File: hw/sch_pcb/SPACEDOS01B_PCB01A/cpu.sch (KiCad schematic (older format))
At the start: 27 parts, among them J19 HEADER_2x01_PARALLEL, J22 HEADER_2x03, J4 HEADER_1x01, J5 HEADER_1x01, J6 HEADER_1x01, J7 HEADER_1x01, U10 ATMEGA1284P-AU, U11 PCF85263A, Y1 16MHz, Y2 ABS07-120-32.768KHZ-T

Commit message: edit
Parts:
- C26, C27, C28, C30, C31, C33, C34, C35, C39, C40, C43, C44, C47: symbol SPACEDOS01A_PCB01A-rescue:C-device-DATALOGGER01A-rescue-CCP2019V01A-rescue -> SPACEDOS01B_PCB01A-rescue:C-device-DATALOGGER01A-rescue-CCP2019V01A-rescue-SPACEDOS01A_PCB01A-rescue
- L1: symbol SPACEDOS01A_PCB01A-rescue:L-device-DATALOGGER01A-rescue-CCP2019V01A-rescue -> SPACEDOS01B_PCB01A-rescue:L-device-DATALOGGER01A-rescue-CCP2019V01A-rescue-SPACEDOS01A_PCB01A-rescue
- R20, R21, R23: symbol SPACEDOS01A_PCB01A-rescue:R-device-DATALOGGER01A-rescue-CCP2019V01A-rescue -> SPACEDOS01B_PCB01A-rescue:R-device-DATALOGGER01A-rescue-CCP2019V01A-rescue-SPACEDOS01A_PCB01A-rescue
- U10: symbol SPACEDOS01A_PCB01A-rescue:ATMEGA1284P-AU-atmel-DATALOGGER01A-rescue-CCP2019V01A-rescue -> SPACEDOS01B_PCB01A-rescue:ATMEGA1284P-AU-atmel-DATALOGGER01A-rescue-CCP2019V01A-rescue-SPACEDOS01A_PCB01A-rescue
- Y2: symbol SPACEDOS01A_PCB01A-rescue:Crystal-device-DATALOGGER01A-rescue-CCP2019V01A-rescue -> SPACEDOS01B_PCB01A-rescue:Crystal-device-DATALOGGER01A-rescue-CCP2019V01A-rescue-SPACEDOS01A_PCB01A-rescue
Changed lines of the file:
@@
 EESchema Schematic File Version 4
-LIBS:SPACEDOS01A_PCB01A-cache
+LIBS:SPACEDOS01B_PCB01A-cache
 EELAYER 26 0
 EELAYER END
@@
 $EndDescr
 $Comp
-L SPACEDOS01A_PCB01A-rescue:ATMEGA1284P-AU-atmel-DATALOGGER01A-rescue-CCP2019V01A-rescue U10
+L SPACEDOS01B_PCB01A-rescue:ATMEGA1284P-AU-atmel-DATALOGGER01A-rescue-CCP2019V01A-rescue-SPACEDOS01A_PCB01A-rescue U10
 U 1 1 5B17AB5A
 P 5850 3200
@@
 	6850 3100 6950 3100
 $Comp
-L SPACEDOS01A_PCB01A-rescue:C-device-DATALOGGER01A-rescue-CCP2019V01A-rescue C40
+L SPACEDOS01B_PCB01A-rescue:C-device-DATALOGGER01A-rescue-CCP2019V01A-rescue-SPACEDOS01A_PCB01A-rescue C40
 U 1 1 5B1D7340
 P 4150 2950
@@
 $EndComp
 $Comp
-L SPACEDOS01A_PCB01A-rescue:C-device-DATALOGGER01A-rescue-CCP2019V01A-rescue C44
+L SPACEDOS01B_PCB01A-rescue:C-device-DATALOGGER01A-rescue-CCP2019V01A-rescue-SPACEDOS01A_PCB01A-rescue C44
 U 1 1 5B1D748A
 P 4600 2950
@@
 	4600 3150 4600 3100
 $Comp
-L SPACEDOS01A_PCB01A-rescue:C-device-DATALOGGER01A-rescue-CCP2019V01A-rescue C43
+L SPACEDOS01B_PCB01A-rescue:C-device-DATALOGGER01A-rescue-CCP2019V01A-rescue-SPACEDOS01A_PCB01A-rescue C43
 U 1 1 5B1E158F
 P 4400 1500
@@
 $EndComp
 $Comp
-L SPACEDOS01A_PCB01A-rescue:R-device-DATALOGGER01A-rescue-CCP2019V01A-rescue R23
+L SPACEDOS01B_PCB01A-rescue:R-device-DATALOGGER01A-rescue-CCP2019V01A-rescue-SPACEDOS01A_PCB01A-rescue R23
 U 1 1 5B1E1A11
 P 4700 1200
@@
 	5650 1150 5650 1000
 $Comp
-L SPACEDOS01A_PCB01A-rescue:C-device-DATALOGGER01A-rescue-CCP2019V01A-rescue C26
+L SPACEDOS01B_PCB01A-rescue:C-device-DATALOGGER01A-rescue-CCP2019V01A-rescue-SPACEDOS01A_PCB01A-rescue C26
 U 1 1 5B1F6794
 P 750 1000
@@
 $EndComp
 $Comp
-L SPACEDOS01A_PCB01A-rescue:C-device-DATALOGGER01A-rescue-CCP2019V01A-rescue C27
+L SPACEDOS01B_PCB01A-rescue:C-device-DATALOGGER01A-rescue-CCP2019V01A-rescue-SPACEDOS01A_PCB01A-rescue C27
 U 1 1 5B1F69A6
 P 1200 1000
@@
 $EndComp
 $Comp
-L SPACEDOS01A_PCB01A-rescue:C-device-DATALOGGER01A-rescue-CCP2019V01A-rescue C28
+L SPACEDOS01B_PCB01A-rescue:C-device-DATALOGGER01A-rescue-CCP2019V01A-rescue-SPACEDOS01A_PCB01A-rescue C28
 U 1 1 5B1F6A02
 P 1650 1000
@@
 $EndComp
 $Comp
-L SPACEDOS01A_PCB01A-rescue:L-device-DATALOGGER01A-rescue-CCP2019V01A-rescue L1
+L SPACEDOS01B_PCB01A-rescue:L-device-DATALOGGER01A-rescue-CCP2019V01A-rescue-SPACEDOS01A_PCB01A-rescue L1
 U 1 1 5B1F6A96
 P 2100 800
@@
 $EndComp
 $Comp
-L SPACEDOS01A_PCB01A-rescue:C-device-DATALOGGER01A-rescue-CCP2019V01A-rescue C31
+L SPACEDOS01B_PCB01A-rescue:C-device-DATALOGGER01A-rescue-CCP2019V01A-rescue-SPACEDOS01A_PCB01A-rescue C31
 U 1 1 5B1F6B7D
 P 2500 1000
@@
 	2500 1200 2500 1150
 $Comp
-L SPACEDOS01A_PCB01A-rescue:C-device-DATALOGGER01A-rescue-CCP2019V01A-rescue C30
+L SPACEDOS01B_PCB01A-rescue:C-device-DATALOGGER01A-rescue-CCP2019V01A-rescue-SPACEDOS01A_PCB01A-rescue C30
 U 1 1 5B2480A8
 P 2400 2600
@@
 $EndComp
 $Comp
-L SPACEDOS01A_PCB01A-rescue:C-device-DATALOGGER01A-rescue-CCP2019V01A-rescue C33
+L SPACEDOS01B_PCB01A-rescue:C-device-DATALOGGER01A-rescue-CCP2019V01A-rescue-SPACEDOS01A_PCB01A-rescue C33
 U 1 1 5B24828C
 P 3000 2600
@@
 TX0
 $Comp
-L SPACEDOS01A_PCB01A-rescue:R-device-DATALOGGER01A-rescue-CCP2019V01A-rescue R20
+L SPACEDOS01B_PCB01A-rescue:R-device-DATALOGGER01A-rescue-CCP2019V01A-rescue-SPACEDOS01A_PCB01A-rescue R20
 U 1 1 5B34D4AA
 P 700 3700
@@
 $EndComp
 $Comp
-L SPACEDOS01A_PCB01A-rescue:R-device-DATALOGGER01A-rescue-CCP2019V01A-rescue R21
+L SPACEDOS01B_PCB01A-rescue:R-device-DATALOGGER01A-rescue-CCP2019V01A-rescue-SPACEDOS01A_PCB01A-rescue R21
 U 1 1 5B34D7C9
 P 900 3700
@@
 	9550 4250 9550 4150
 $Comp
-L SPACEDOS01A_PCB01A-rescue:Crystal-device-DATALOGGER01A-rescue-CCP2019V01A-rescue Y2
+L SPACEDOS01B_PCB01A-rescue:Crystal-device-DATALOGGER01A-rescue-CCP2019V01A-rescue-SPACEDOS01A_PCB01A-rescue Y2
 U 1 1 5B36B778
 P 8750 4650
@@
 	8550 5400 9050 5400
 $Comp
-L SPACEDOS01A_PCB01A-rescue:C-device-DATALOGGER01A-rescue-CCP2019V01A-rescue C47
+L SPACEDOS01B_PCB01A-rescue:C-device-DATALOGGER01A-rescue-CCP2019V01A-rescue-SPACEDOS01A_PCB01A-rescue C47
 U 1 1 5B38BB8A
 P 10800 5850
@@
 $EndComp
 $Comp
-L SPACEDOS01A_PCB01A-rescue:C-device-DATALOGGER01A-rescue-CCP2019V01A-rescue C34
+L SPACEDOS01B_PCB01A-rescue:C-device-DATALOGGER01A-rescue-CCP2019V01A-rescue-SPACEDOS01A_PCB01A-rescue C34
 U 1 1 5B36FE27
 P 3100 1000
@@
 	3100 800  3100 850
 $Comp
-L SPACEDOS01A_PCB01A-rescue:C-device-DATALOGGER01A-rescue-CCP2019V01A-rescue C35
+L SPACEDOS01B_PCB01A-rescue:C-device-DATALOGGER01A-rescue-CCP2019V01A-rescue-SPACEDOS01A_PCB01A-rescue C35
 U 1 1 5B38C9AC
 P 3550 1000
@@
 	3550 800  3550 850
 $Comp
-L SPACEDOS01A_PCB01A-rescue:C-device-DATALOGGER01A-rescue-CCP2019V01A-rescue C39
+L SPACEDOS01B_PCB01A-rescue:C-device-DATALOGGER01A-rescue-CCP2019V01A-rescue-SPACEDOS01A_PCB01A-rescue C39
 U 1 1 5B3A9D6D
 P 4050 1000

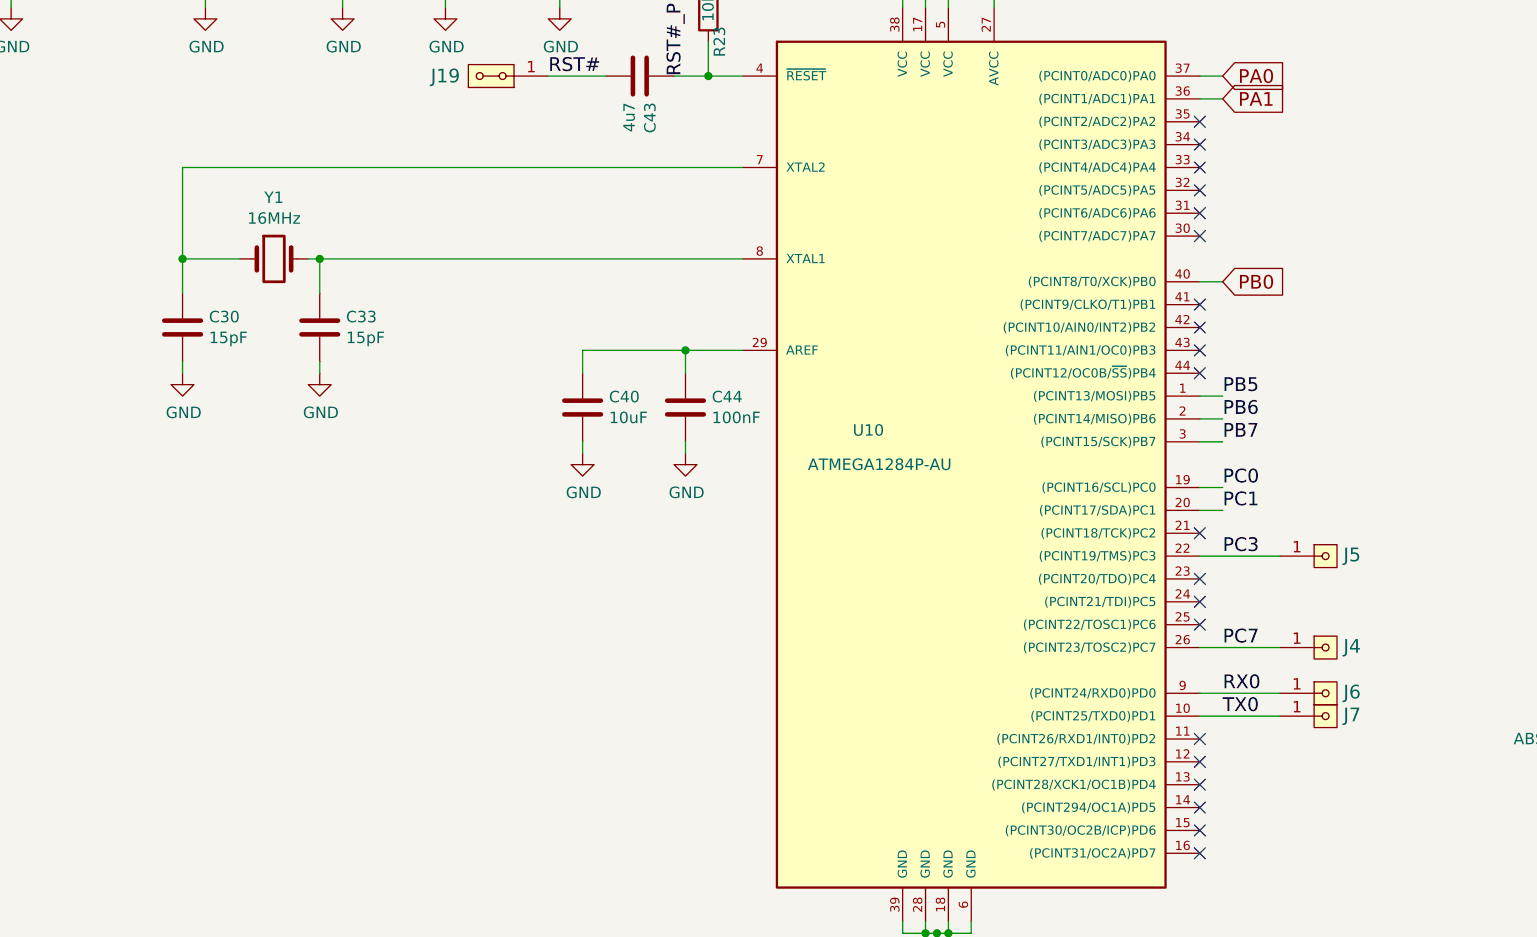
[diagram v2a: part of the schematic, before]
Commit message: edit
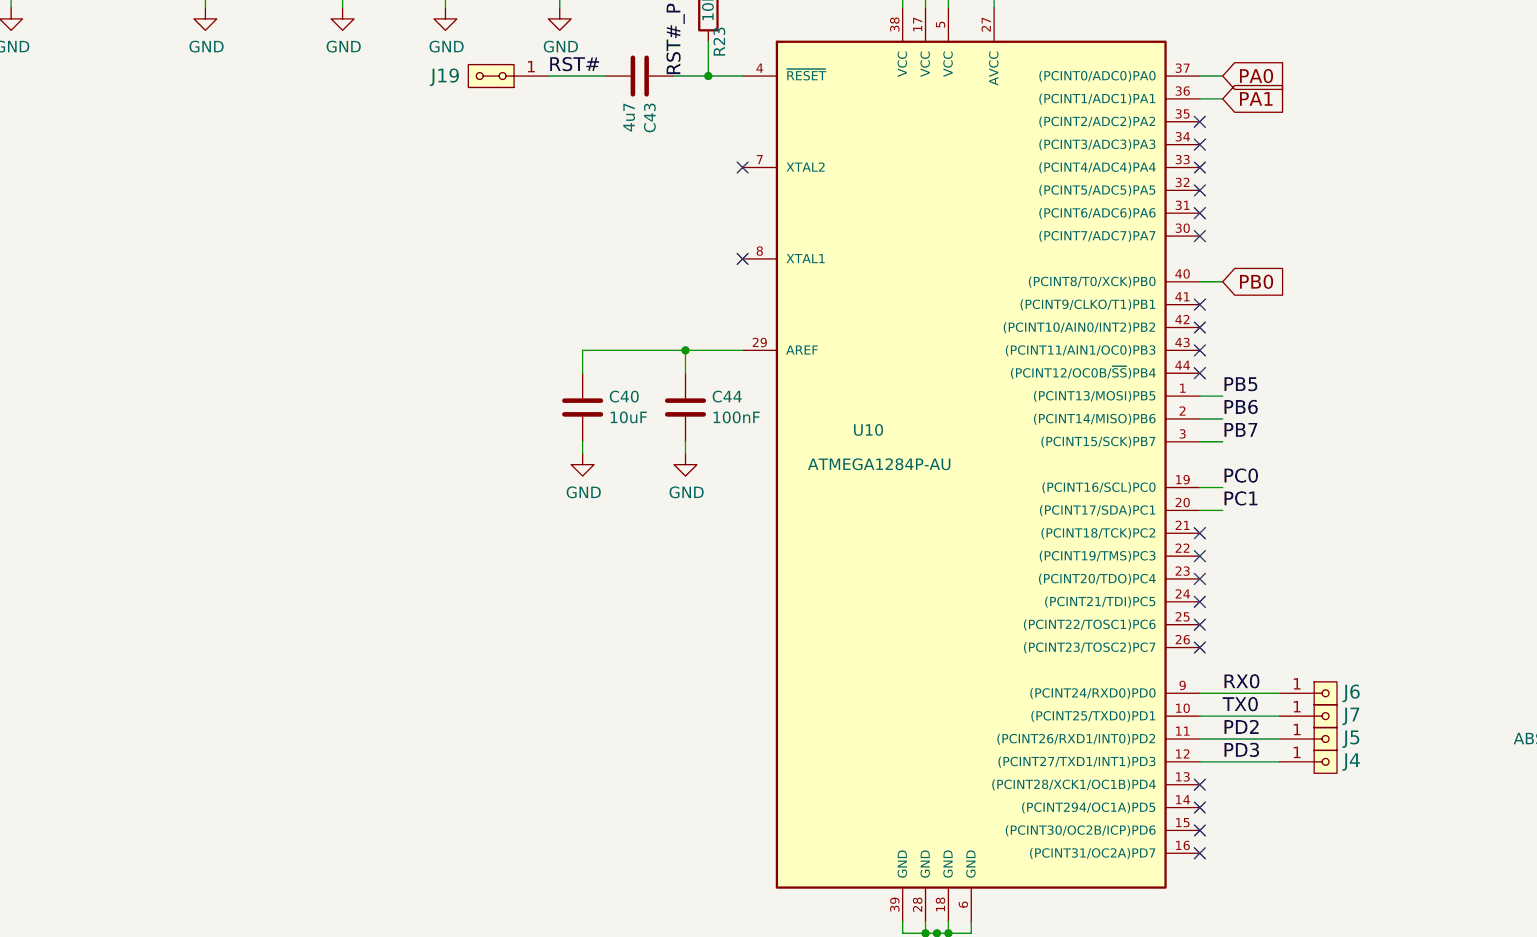
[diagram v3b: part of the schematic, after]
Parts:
- removed C30, C33: 15pF, Mlab_R:SMD-0805, symbol SPACEDOS01B_PCB01A-rescue:C-device-DATALOGGER01A-rescue-CCP2019V01A-rescue-SPAC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
- removed Y1: 16MHz, Mlab_XTAL:Crystal_HC49-4H_Vertical, symbol Device:Crystal
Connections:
- net PD2: now reaches U10.11 ((PCINT26/RXD1/INT0)PD2)
- net PD2: now also J5.1
- net PD3: now reaches U10.12 ((PCINT27/TXD1/INT1)PD3)
- net PD3: now also J4.1
- net PC3: no longer names the net of U10.22 ((PCINT19/TMS)PC3)
- net PC3: no longer J5.1
- net PC7: no longer names the net of U10.26 ((PCINT23/TOSC2)PC7)
- net PC7: no longer J4.1
- no-connect marks 23 -> 25
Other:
- moved on the sheet: J4, J5
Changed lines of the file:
@@
 	2500 1200 2500 1150
-$Comp
-L SPACEDOS01B_PCB01A-rescue:C-device-DATALOGGER01A-rescue-CCP2019V01A-rescue-SPACEDOS01A_PCB01A-rescue C30
-U 1 1 5B2480A8
-P 2400 2600
-F 0 "C30" H 2515 2646 50  0000 L CNN
-F 1 "15pF" H 2515 2555 50  0000 L CNN
-F 2 "Mlab_R:SMD-0805" H 2438 2450 50  0001 C CNN
-F 3 "" H 2400 2600 50  0001 C CNN
-	1    2400 2600
-	1    0    0    -1
-$EndComp
-$Comp
-L SPACEDOS01B_PCB01A-rescue:C-device-DATALOGGER01A-rescue-CCP2019V01A-rescue-SPACEDOS01A_PCB01A-rescue C33
-U 1 1 5B24828C
-P 3000 2600
-F 0 "C33" H 3115 2646 50  0000 L CNN
-F 1 "15pF" H 3115 2555 50  0000 L CNN
-F 2 "Mlab_R:SMD-0805" H 3038 2450 50  0001 C CNN
-F 3 "" H 3000 2600 50  0001 C CNN
-	1    3000 2600
-	1    0    0    -1
-$EndComp
-$Comp
-L power:GND #PWR0126
-U 1 1 5B248495
-P 3000 2800
-F 0 "#PWR0126" H 3000 2550 50  0001 C CNN
-F 1 "GND" H 3005 2627 50  0000 C CNN
-F 2 "" H 3000 2800 50  0001 C CNN
-F 3 "" H 3000 2800 50  0001 C CNN
-	1    3000 2800
-	1    0    0    -1
-$EndComp
-$Comp
-L power:GND #PWR0127
-U 1 1 5B2484F8
-P 2400 2800
-F 0 "#PWR0127" H 2400 2550 50  0001 C CNN
-F 1 "GND" H 2405 2627 50  0000 C CNN
-F 2 "" H 2400 2800 50  0001 C CNN
-F 3 "" H 2400 2800 50  0001 C CNN
-	1    2400 2800
-	1    0    0    -1
-$EndComp
-Wire Wire Line
-	2400 2800 2400 2750
-Wire Wire Line
-	3000 2800 3000 2750
-Wire Wire Line
-	2650 2300 2400 2300
-Connection ~ 2400 2300
-Wire Wire Line
-	2400 2300 2400 2450
-Wire Wire Line
-	3000 2300 2950 2300
-Wire Wire Line
-	3000 2300 3000 2450
-Connection ~ 3000 2300
-Wire Wire Line
-	2400 1900 2400 2300
 $Comp
 L power:GND #PWR0129
@@
 	6150 6100 6400 6100
 $Comp
-L Device:Crystal Y1
-U 1 1 5B257330
-P 2800 2300
-F 0 "Y1" H 2800 2568 50  0000 C CNN
-F 1 "16MHz" H 2800 2477 50  0000 C CNN
-F 2 "Mlab_XTAL:Crystal_HC49-4H_Vertical" H 2800 2300 50  0001 C CNN
-F 3 "~" H 2800 2300 50  0001 C CNN
-	1    2800 2300
-	1    0    0    -1
-$EndComp
-$Comp
 L SPACEDOS01B_PCB01A-rescue:C-device-DATALOGGER01A-rescue-CCP2019V01A-rescue-SPACEDOS01A_PCB01A-rescue C34
 U 1 1 5B36FE27
@@
 Wire Wire Line
 	4150 2700 4600 2700
-Wire Wire Line
-	2400 1900 4850 1900
-Wire Wire Line
-	3000 2300 4850 2300
 $Comp
 L power:+3.3V #PWR0118
@@
 	1    0    0    -1
 $EndComp
-Wire Wire Line
-	6850 3600 7200 3600
 NoConn ~ 10300 5600
 NoConn ~ 10300 5400
@@
 NoConn ~ 6850 4700
 NoConn ~ 6850 4600
-NoConn ~ 6850 4500
-NoConn ~ 6850 4400
+NoConn ~ 6850 4000
+NoConn ~ 6850 3600
 NoConn ~ 6850 3900
 NoConn ~ 6850 3800
@@
 NoConn ~ 6850 1800
 NoConn ~ 6850 1700
-Text Label 6950 4000 0    60   ~ 0
-PC7
-Text Label 6950 3600 0    60   ~ 0
-PC3
+Text Label 6950 4500 0    60   ~ 0
+PD3
+Text Label 6950 4400 0    60   ~ 0
+PD2
 $Comp
 L MLAB_HEADER:HEADER_1x01 J4
 U 1 1 5C6A22D0
-P 7400 4000
-F 0 "J4" H 7478 4005 60  0000 L CNN
-F 1 "HEADER_1x01" H 7478 3952 60  0001 L CNN
-F 2 "Mlab_Pin_Headers:Straight_1x01" H 7400 4000 60  0001 C CNN
-F 3 "" H 7400 4000 60  0000 C CNN
-	1    7400 4000
+P 7400 4500
+F 0 "J4" H 7478 4505 60  0000 L CNN
+F 1 "HEADER_1x01" H 7478 4452 60  0001 L CNN
+F 2 "Mlab_Pin_Headers:Straight_1x01" H 7400 4500 60  0001 C CNN
+F 3 "" H 7400 4500 60  0000 C CNN
+	1    7400 4500
 	1    0    0    -1
 $EndComp
@@
 L MLAB_HEADER:HEADER_1x01 J5
 U 1 1 5C6A319F
-P 7400 3600
-F 0 "J5" H 7478 3605 60  0000 L CNN
-F 1 "HEADER_1x01" H 7478 3552 60  0001 L CNN
-F 2 "Mlab_Pin_Headers:Straight_1x01" H 7400 3600 60  0001 C CNN
-F 3 "" H 7400 3600 60  0000 C CNN
-	1    7400 3600
+P 7400 4400
+F 0 "J5" H 7478 4405 60  0000 L CNN
+F 1 "HEADER_1x01" H 7478 4352 60  0001 L CNN
+F 2 "Mlab_Pin_Headers:Straight_1x01" H 7400 4400 60  0001 C CNN
+F 3 "" H 7400 4400 60  0000 C CNN
+	1    7400 4400
 	1    0    0    -1
 $EndComp
@@
 	1    0    0    -1
 $EndComp
-Wire Wire Line
-	6850 4000 7200 4000
 NoConn ~ 6850 2800
 NoConn ~ 6850 3500
@@
 Wire Wire Line
 	6850 2400 6950 2400
+Wire Wire Line
+	6850 4400 7200 4400
+Wire Wire Line
+	6850 4500 7200 4500
+NoConn ~ 4850 1900
+NoConn ~ 4850 2300
 $EndSCHEMATC
